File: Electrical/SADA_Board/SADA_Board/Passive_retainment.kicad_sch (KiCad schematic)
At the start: 20 parts, among them J11 105431-1202, J12 105431-1202, U10 Si1442DH, U8 TPS62867RQYR, U9 Si1442DH

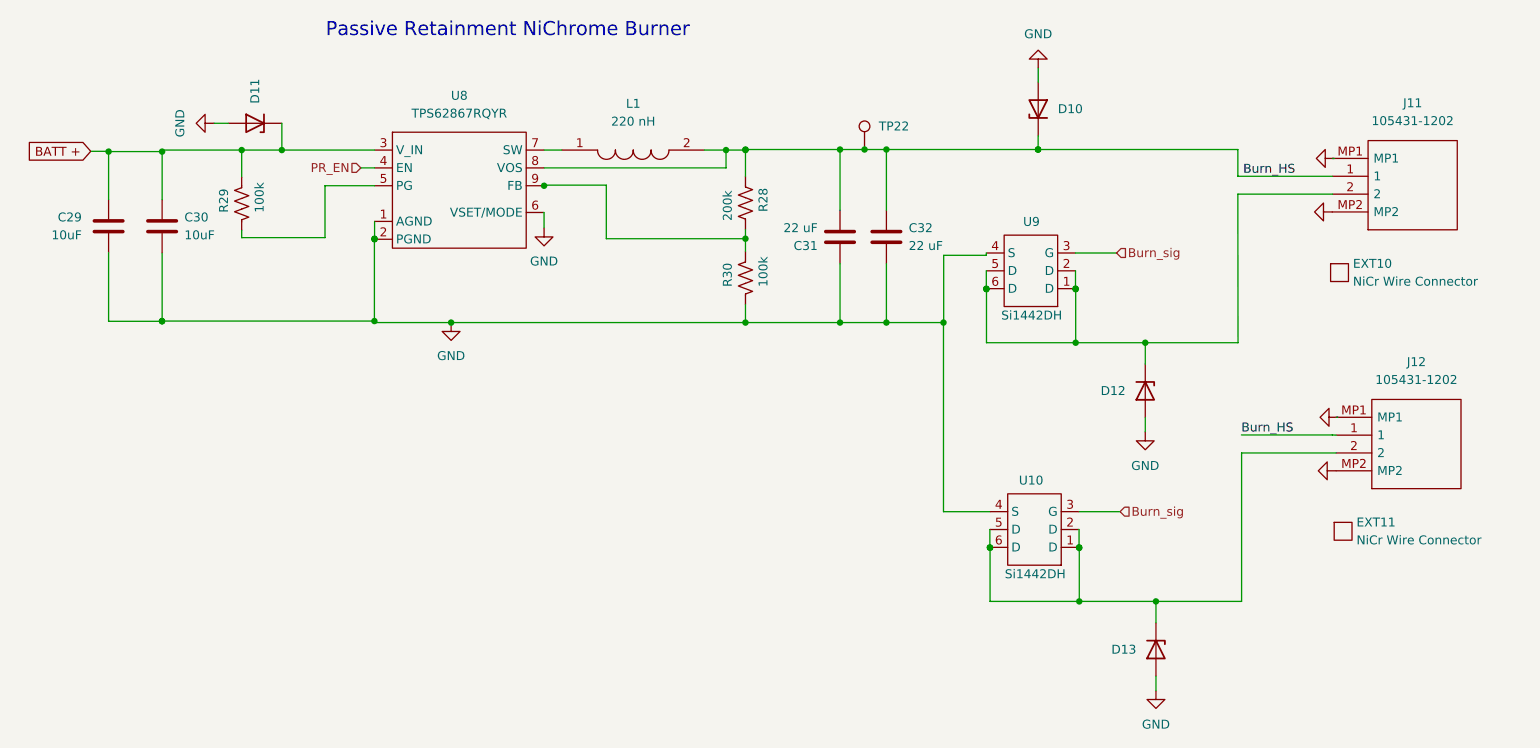
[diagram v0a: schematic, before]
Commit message: ESD changes
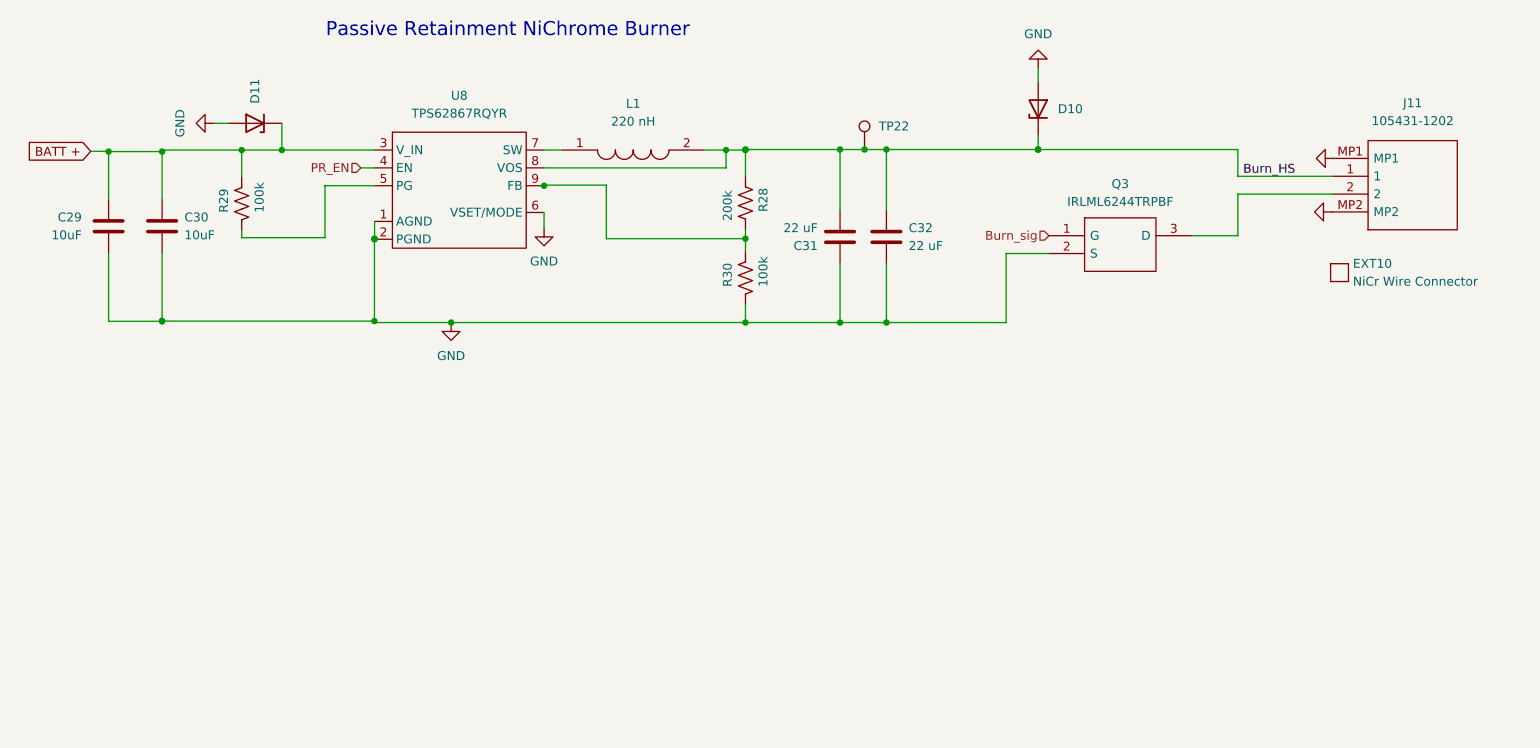
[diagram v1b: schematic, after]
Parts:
- removed D12, D13: TVS, symbol Diode:ESD5Zxx
- removed EXT11: NiCr Wire Connector, 0_custom:EXT_no_footprint, symbol 0_custom:{lt}name{gt}
- removed J12: 105431-1202, Miles Added:1054311202, symbol molex_105431-1202:105431-1202
- removed U10, U9: Si1442DH, Package_TO_SOT_SMD:SOT-363_SC-70-6, symbol 0_custom:Si1442DH
- added Q3: IRLML6244TRPBF, SOT95P237X112-3N, symbol IRLML6244TRPBF:IRLML6244TRPBF
- D10, D11: footprint (none) -> Diode_SMD:D_0402_1005Metric
- TP22: footprint TestPoint:TestPoint_Pad_D1.5mm -> TestPoint:TestPoint_Pad_D1.0mm
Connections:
- net Burn_sig: now also Q3.1 (G)
- net GND: now also Q3.2 (S)
- net at J11.2: now also Q3.3 (D)
